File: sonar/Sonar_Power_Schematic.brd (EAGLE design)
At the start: 100 x 80 mm, 34 parts, among them U1 LT3471', U2 LT3045, U3 LT3045, U4 LT1175

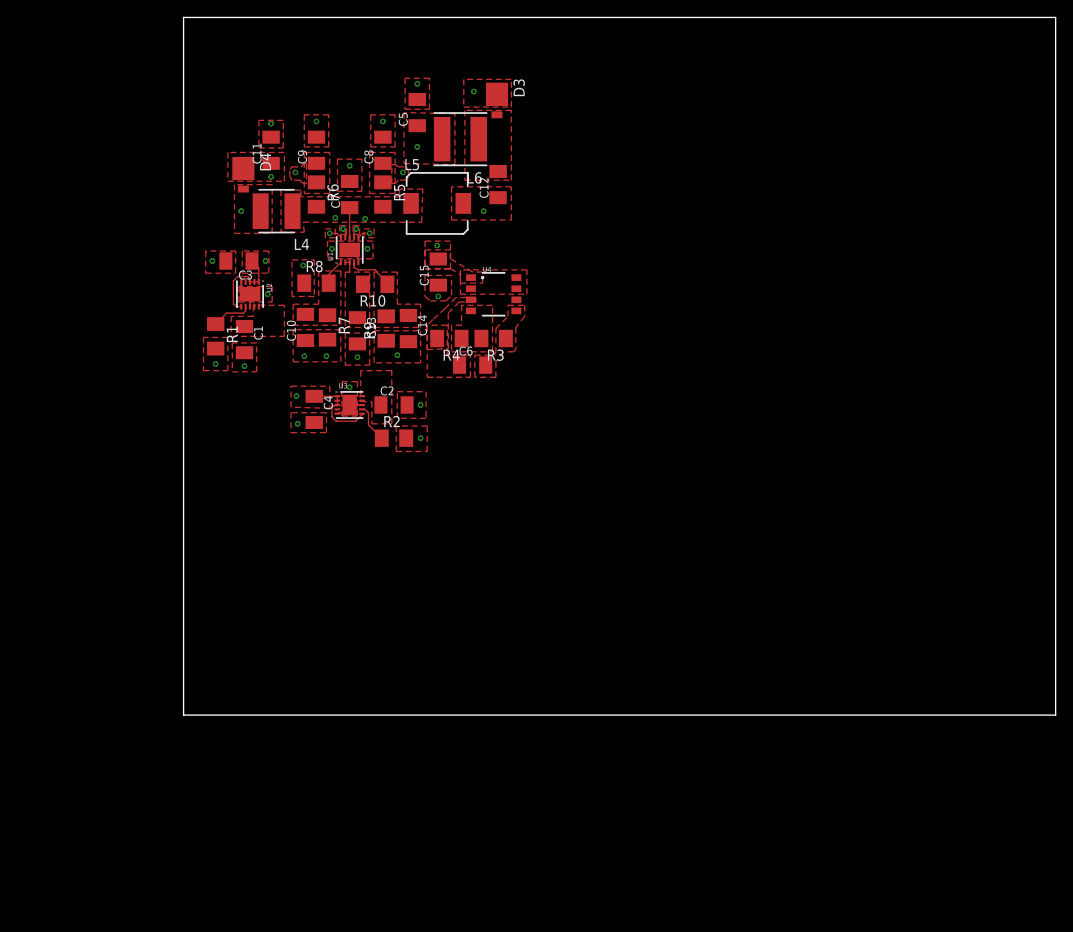
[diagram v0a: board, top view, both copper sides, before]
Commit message: DRC updated
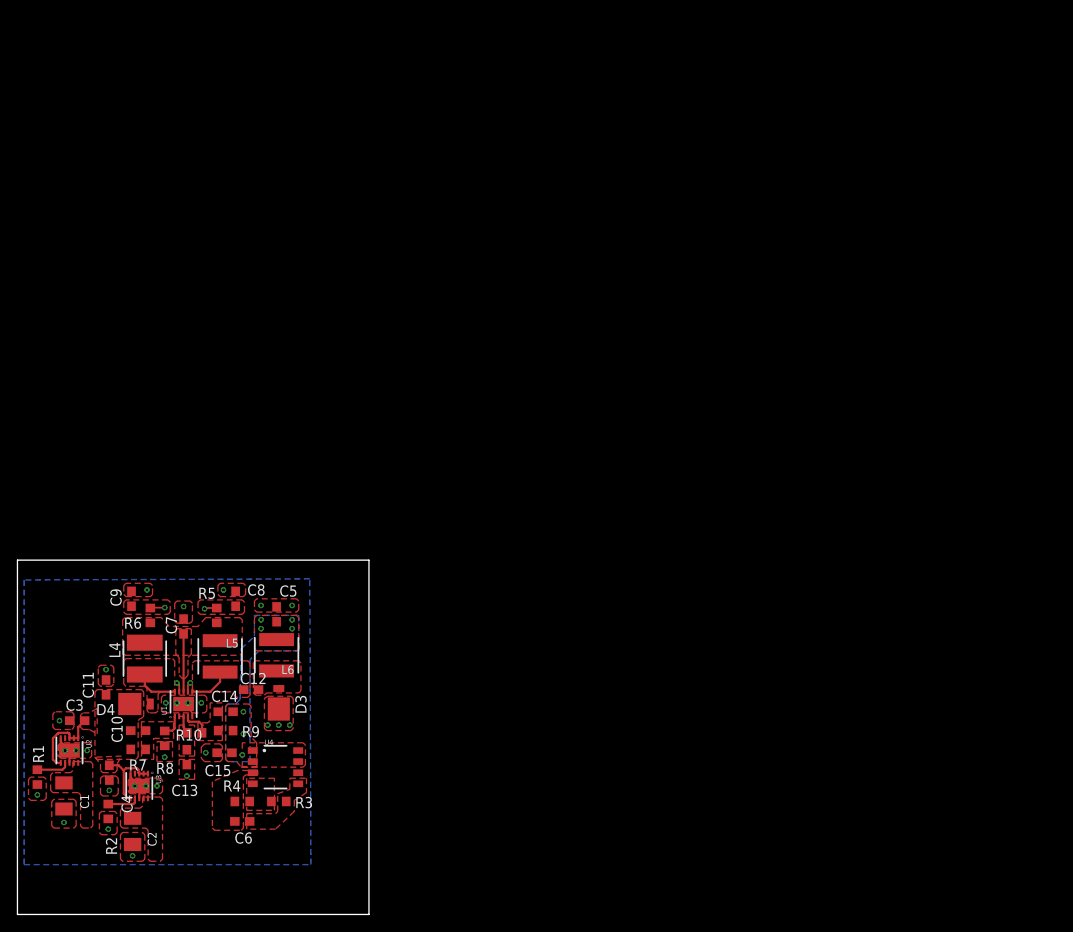
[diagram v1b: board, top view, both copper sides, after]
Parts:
- C10, C11, C12, C13, C14, C15, C5, C6, C7, C8, C9: device adafruit:C1206K -> adafruit:C0603
- C3, C4: value 10uF -> 4.7uF; device adafruit:C1206K -> adafruit:C0603
- L5: device Moira:NS7X7 -> Moira:NS5X5
- L6: device Moira:NS6X6 -> Moira:NS5X5
- R1, R10, R2, R3, R4, R5, R6, R7, R8, R9: device adafruit:M3216 -> adafruit:R0603
- moved D3 73.5 mm to (10.9, 1.40), turned to 90 degrees
- moved C12 64.5 mm to (7.75, 2.92), turned to 0 degrees
- moved C11 64.4 mm to (-8.89, 3.17)
- moved L6 62.8 mm to (10.7, 6.86), turned to 90 degrees
- moved D4 61.9 mm to (-5.46, 1.27), turned to 0 degrees
- moved C15 60.3 mm to (4.70, -4.32), turned to 0 degrees
- moved C5 59.7 mm to (10.7, 11.6)
- moved U4 59.7 mm to (10.5, -5.97)
- moved C6 58.6 mm to (6.73, -12.2)
- moved R3 58.5 mm to (10.9, -9.91)
- moved R4 58.2 mm to (6.73, -9.91)
- moved L5 57.6 mm to (4.19, 6.73), turned to 270 degrees
- moved C2 57.4 mm to (-5.84, -13.3), turned to 270 degrees
- moved C1 56.3 mm to (-13.7, -9.27)
- moved U2 56.3 mm to (-13.1, -4.06)
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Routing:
- net SS1: track 1.11 -> 12.0 mm
- net SS2: track 1.11 -> 12.0 mm
- net N$17: track 1.49 -> 4.98 mm, vias 2 -> 0
- net N$20: track 1.49 -> 4.78 mm, vias 2 -> 0
- net VIN: track 3.44 -> 6.63 mm, vias 2 -> 0
- net N$26: track 5.44 -> 3.26 mm
- net 7.5V: track 19.5 -> 18.4 mm, vias 5 -> 0
- net VREF: track 1.63 -> 2.51 mm
- net N$4: track 4.46 -> 3.61 mm
- net N$6: track 4.55 -> 3.79 mm
- net GND: vias 19 -> 28
- added copper zone on layer 16, net -7.5V
- added copper zone on layer 16, net GND
- removed copper zone on layer 4, net -7.5V
- removed copper zone on layer 4, net 7.5V
- removed copper zone on layer 4, net GND
- removed copper zone on layer 3, net N$17
- removed copper zone on layer 3, net N$20
- removed copper zone on layer 3, net SS1
- removed copper zone on layer 3, net SS2
- removed copper zone on layer 4, net VIN
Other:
- board size 100 x 80 mm -> 40.3 x 40.6 mm
